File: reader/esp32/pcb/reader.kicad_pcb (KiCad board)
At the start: 2 copper layers, 96.5 x 30.1 mm, 28 parts, among them J1 Conn_01x06, J2 Conn_01x02, J3 Conn_01x04, J4 Conn_01x02, Q1 MMBT3904, Q2 MMBT3904, U1 ESP32-WROOM-32U, U2 RF125-PS, U3 CH340C, U4 74LVC1T45, U5 AMS1117-3.3

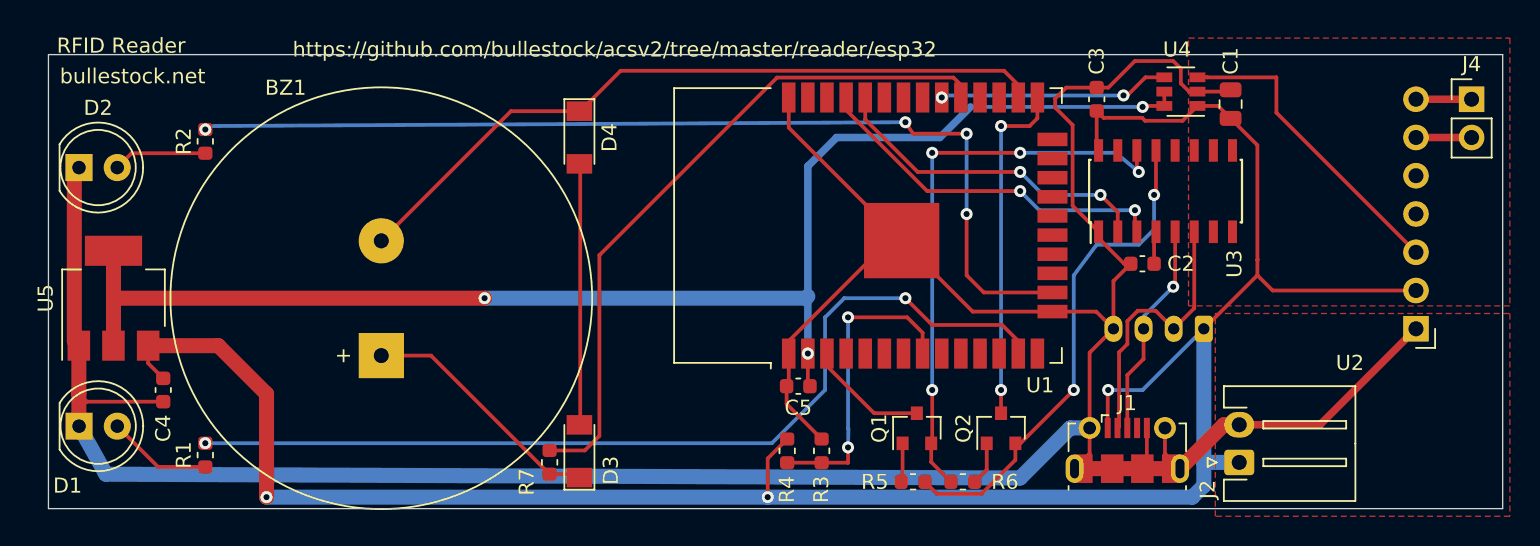
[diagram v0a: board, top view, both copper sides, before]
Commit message: Cleanup.
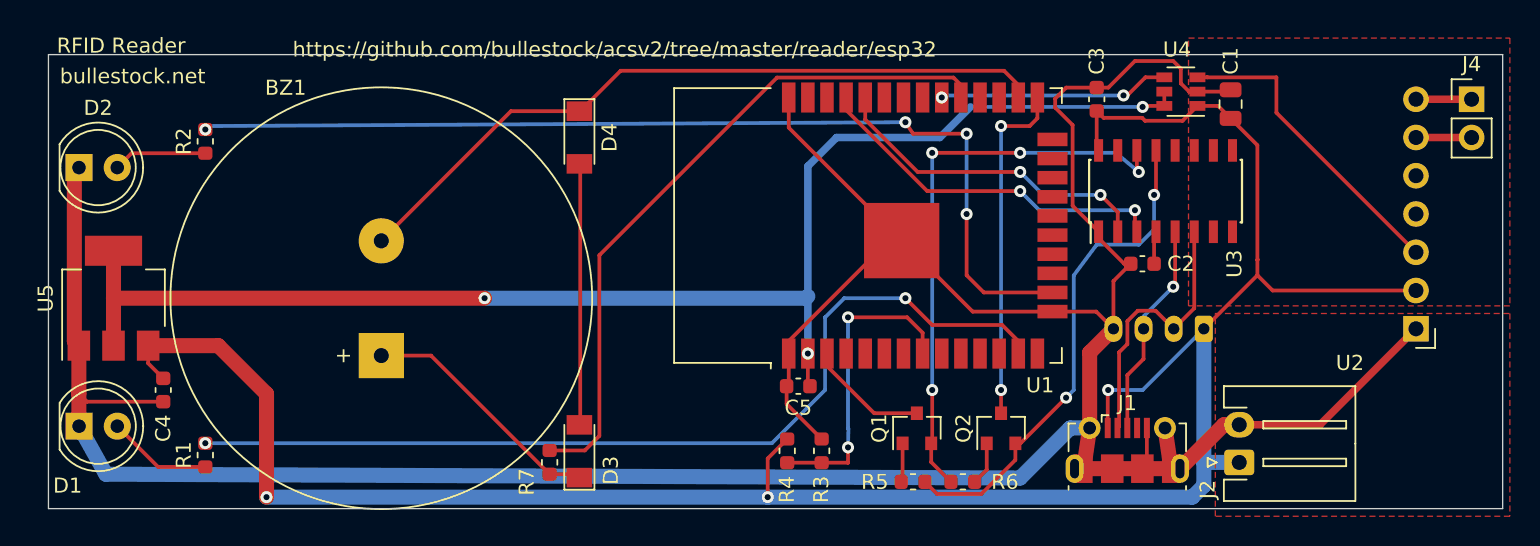
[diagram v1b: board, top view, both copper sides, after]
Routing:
- net GND: track 221.6 -> 211.4 mm
- net ESP_TX: track 24.2 -> 23.2 mm
- net RED: track 62.8 -> 62.0 mm
- net EN: track 8.10 -> 7.27 mm
- net BUZ2: track 48.2 -> 47.4 mm
- net BUZ1: track 45.6 -> 44.8 mm
